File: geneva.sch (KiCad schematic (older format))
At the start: 8 parts, among them J1 USB_B_Micro

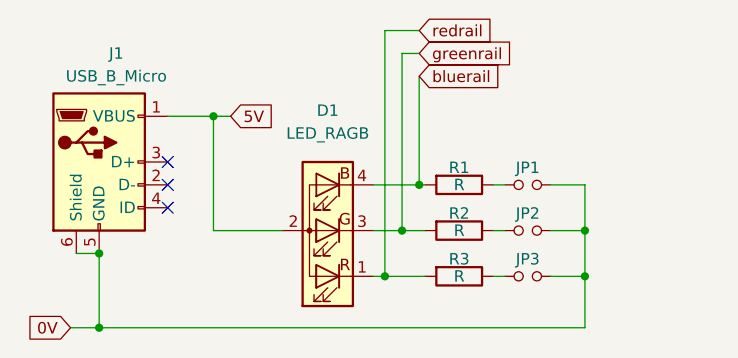
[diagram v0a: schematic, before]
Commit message: Updated nets
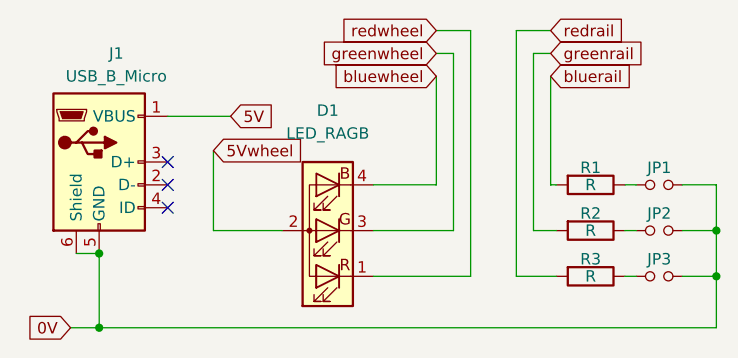
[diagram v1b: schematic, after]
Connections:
- net 5V: no longer D1.2 (A)
- net bluerail: no longer D1.4 (BK)
- net greenrail: no longer D1.3 (GK)
- net redrail: no longer D1.1 (RK)
- new net 5Vwheel: D1.2 (A)
- new net bluewheel: D1.4 (BK)
- new net greenwheel: D1.3 (GK)
- new net redwheel: D1.1 (RK)
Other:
- moved on the sheet: JP1, JP2, JP3, R1, R2, R3
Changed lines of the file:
@@
 	1525 6250 1625 6250
 Connection ~ 1625 6250
-Wire Wire Line
-	1925 5650 2125 5650
 Text GLabel 1500 6575 0    50   Input ~ 0
 0V
@@
 L Device:R R1
 U 1 1 5E1E4A47
-P 3200 5950
-F 0 "R1" V 3125 5950 50  0000 C CNN
-F 1 "R" V 3200 5950 50  0000 C CNN
-F 2 "Resistor_THT:R_Axial_DIN0204_L3.6mm_D1.6mm_P7.62mm_Horizontal" V 3130 5950 50  0001 C CNN
-F 3 "~" H 3200 5950 50  0001 C CNN
-	1    3200 5950
+P 3775 5950
+F 0 "R1" V 3700 5950 50  0000 C CNN
+F 1 "R" V 3775 5950 50  0000 C CNN
+F 2 "Resistor_THT:R_Axial_DIN0204_L3.6mm_D1.6mm_P7.62mm_Horizontal" V 3705 5950 50  0001 C CNN
+F 3 "~" H 3775 5950 50  0001 C CNN
+	1    3775 5950
 	0    1    1    0
 $EndComp
@@
 L Device:R R2
 U 1 1 5E1E4F47
-P 3200 6150
-F 0 "R2" V 3125 6150 50  0000 C CNN
-F 1 "R" V 3200 6150 50  0000 C CNN
-F 2 "Resistor_THT:R_Axial_DIN0204_L3.6mm_D1.6mm_P7.62mm_Horizontal" V 3130 6150 50  0001 C CNN
-F 3 "~" H 3200 6150 50  0001 C CNN
-	1    3200 6150
+P 3775 6150
+F 0 "R2" V 3700 6150 50  0000 C CNN
+F 1 "R" V 3775 6150 50  0000 C CNN
+F 2 "Resistor_THT:R_Axial_DIN0204_L3.6mm_D1.6mm_P7.62mm_Horizontal" V 3705 6150 50  0001 C CNN
+F 3 "~" H 3775 6150 50  0001 C CNN
+	1    3775 6150
 	0    1    1    0
 $EndComp
@@
 L Device:R R3
 U 1 1 5E1E529E
-P 3200 6350
-F 0 "R3" V 3125 6350 50  0000 C CNN
-F 1 "R" V 3200 6350 50  0000 C CNN
-F 2 "Resistor_THT:R_Axial_DIN0204_L3.6mm_D1.6mm_P7.62mm_Horizontal" V 3130 6350 50  0001 C CNN
-F 3 "~" H 3200 6350 50  0001 C CNN
-	1    3200 6350
+P 3775 6350
+F 0 "R3" V 3700 6350 50  0000 C CNN
+F 1 "R" V 3775 6350 50  0000 C CNN
+F 2 "Resistor_THT:R_Axial_DIN0204_L3.6mm_D1.6mm_P7.62mm_Horizontal" V 3705 6350 50  0001 C CNN
+F 3 "~" H 3775 6350 50  0001 C CNN
+	1    3775 6350
 	0    1    1    0
 $EndComp
@@
 L Device:Jumper_NO_Small JP1
 U 1 1 5E1E5871
-P 3500 5950
-F 0 "JP1" H 3500 6025 50  0000 C CNN
-F 1 "Jumper_NO_Small" H 3500 6050 50  0001 C CNN
-F 2 "geneva:jumper" H 3500 5950 50  0001 C CNN
-F 3 "~" H 3500 5950 50  0001 C CNN
-	1    3500 5950
+P 4075 5950
+F 0 "JP1" H 4075 6025 50  0000 C CNN
+F 1 "Jumper_NO_Small" H 4075 6050 50  0001 C CNN
+F 2 "geneva:jumper" H 4075 5950 50  0001 C CNN
+F 3 "~" H 4075 5950 50  0001 C CNN
+	1    4075 5950
 	1    0    0    -1
 $EndComp
@@
 L Device:Jumper_NO_Small JP2
 U 1 1 5E1E5EA6
-P 3500 6150
-F 0 "JP2" H 3500 6225 50  0000 C CNN
-F 1 "Jumper_NO_Small" H 3500 6250 50  0001 C CNN
-F 2 "geneva:jumper" H 3500 6150 50  0001 C CNN
-F 3 "~" H 3500 6150 50  0001 C CNN
-	1    3500 6150
+P 4075 6150
+F 0 "JP2" H 4075 6225 50  0000 C CNN
+F 1 "Jumper_NO_Small" H 4075 6250 50  0001 C CNN
+F 2 "geneva:jumper" H 4075 6150 50  0001 C CNN
+F 3 "~" H 4075 6150 50  0001 C CNN
+	1    4075 6150
 	1    0    0    -1
 $EndComp
@@
 L Device:Jumper_NO_Small JP3
 U 1 1 5E1E630C
-P 3500 6350
-F 0 "JP3" H 3500 6425 50  0000 C CNN
-F 1 "Jumper_NO_Small" H 3500 6450 50  0001 C CNN
-F 2 "geneva:jumper" H 3500 6350 50  0001 C CNN
-F 3 "~" H 3500 6350 50  0001 C CNN
-	1    3500 6350
+P 4075 6350
+F 0 "JP3" H 4075 6425 50  0000 C CNN
+F 1 "Jumper_NO_Small" H 4075 6450 50  0001 C CNN
+F 2 "geneva:jumper" H 4075 6350 50  0001 C CNN
+F 3 "~" H 4075 6350 50  0001 C CNN
+	1    4075 6350
 	1    0    0    -1
 $EndComp
@@
 	2425 6150 2125 6150
 Wire Wire Line
-	2125 6150 2125 5650
-Connection ~ 2125 5650
+	4175 5950 4325 5950
 Wire Wire Line
-	2125 5650 2200 5650
+	4325 5950 4325 6150
 Wire Wire Line
-	3600 5950 3750 5950
+	4325 6150 4175 6150
 Wire Wire Line
-	3750 5950 3750 6150
+	4325 6150 4325 6350
 Wire Wire Line
-	3750 6150 3600 6150
+	4325 6350 4175 6350
+Connection ~ 4325 6150
 Wire Wire Line
-	3750 6150 3750 6350
-Wire Wire Line
-	3750 6350 3600 6350
-Connection ~ 3750 6150
-Wire Wire Line
-	3750 6350 3750 6575
-Wire Wire Line
-	3750 6575 1625 6575
-Connection ~ 3750 6350
+	4325 6350 4325 6575
+Connection ~ 4325 6350
 Wire Wire Line
 	1625 6250 1625 6575
@@
 Connection ~ 1625 6575
 Wire Wire Line
-	2825 5950 3025 5950
+	3925 6350 3975 6350
 Wire Wire Line
-	2825 6150 2950 6150
+	3975 6150 3925 6150
 Wire Wire Line
-	2825 6350 2875 6350
-Wire Wire Line
-	3350 6350 3400 6350
-Wire Wire Line
-	3400 6150 3350 6150
-Wire Wire Line
-	3350 5950 3400 5950
-Text GLabel 3025 5275 2    50   Input ~ 0
+	3925 5950 3975 5950
+Text GLabel 3600 5275 2    50   Input ~ 0
 redrail
-Text GLabel 3025 5375 2    50   Input ~ 0
+Text GLabel 3600 5375 2    50   Input ~ 0
 greenrail
-Text GLabel 3025 5475 2    50   Input ~ 0
+Text GLabel 3600 5475 2    50   Input ~ 0
 bluerail
 Wire Wire Line
-	3025 5475 3025 5950
-Connection ~ 3025 5950
+	3600 5475 3600 5950
 Wire Wire Line
-	3025 5950 3050 5950
+	3600 5950 3625 5950
 Wire Wire Line
-	3025 5375 2950 5375
+	3600 5375 3525 5375
 Wire Wire Line
-	2950 5375 2950 6150
-Connection ~ 2950 6150
+	3525 5375 3525 6150
 Wire Wire Line
-	2950 6150 3050 6150
+	3525 6150 3625 6150
 Wire Wire Line
-	3025 5275 2875 5275
+	3600 5275 3450 5275
 Wire Wire Line
-	2875 5275 2875 6350
-Connection ~ 2875 6350
+	3450 5275 3450 6350
 Wire Wire Line
-	2875 6350 3050 6350
+	3450 6350 3625 6350
+Wire Wire Line
+	1625 6575 4325 6575
+Wire Wire Line
+	2825 6350 3250 6350
+Wire Wire Line
+	3250 6350 3250 5275
+Text GLabel 3100 5275 0    50   Input ~ 0
+redwheel
+Wire Wire Line
+	3100 5275 3250 5275
+Text GLabel 3100 5375 0    50   Input ~ 0
+greenwheel
+Text GLabel 3100 5475 0    50   Input ~ 0
+bluewheel
+Wire Wire Line
+	3100 5375 3175 5375
+Wire Wire Line
+	3175 5375 3175 6150
+Wire Wire Line
+	3175 6150 2825 6150
+Wire Wire Line
+	3100 5475 3100 5950
+Wire Wire Line
+	3100 5950 2825 5950
+Wire Wire Line
+	1925 5650 2200 5650
+Text GLabel 2125 5800 2    50   Input ~ 0
+5Vwheel
+Wire Wire Line
+	2125 5800 2125 6150
 $EndSCHEMATC
